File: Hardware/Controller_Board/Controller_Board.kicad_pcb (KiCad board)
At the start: 6 copper layers, 85 x 85 mm, 261 parts, among them J601 USB-C, Q101 DMN2400UFB-7, SW301 Reset, U101 TPS82084, U102 LT8645S, U103 TDS5311P, U104 TPS82084, U105 TPS82084, U106 XT30, U201 XC7A35T-CSG324, U301 IS25LP256D, U401 FT232H, U402 93LC56B, U501 FT232H, U502 93LC56B, U601 ESD122, U602 USB2512B, U701 RJ45, U702 RJ45, U703 RJ45, U704 TPD4E02B04, U705 TPD4E02B04, U706 TPD4E02B04, U710 RJ45, U711 RJ45, U712 RJ45, U713 TPD4E02B04, U714 TPD4E02B04, U715 TPD4E02B04, U716 RJ45, U717 RJ45, U718 RJ45, U719 TPD4E02B04, U720 TPD4E02B04, U721 TPD4E02B04, U722 TPD4E02B04, U723 TPD4E02B04, U724 TPD4E02B04, U725 TPD4E02B04, U726 TPD4E02B04, U727 TPD4E02B04, U728 TPD4E02B04, U729 TPD4E02B04, U730 TPD4E02B04, Y1 24MHz, Y2 12MHz, Y3 12MHz, Y301 12MHz

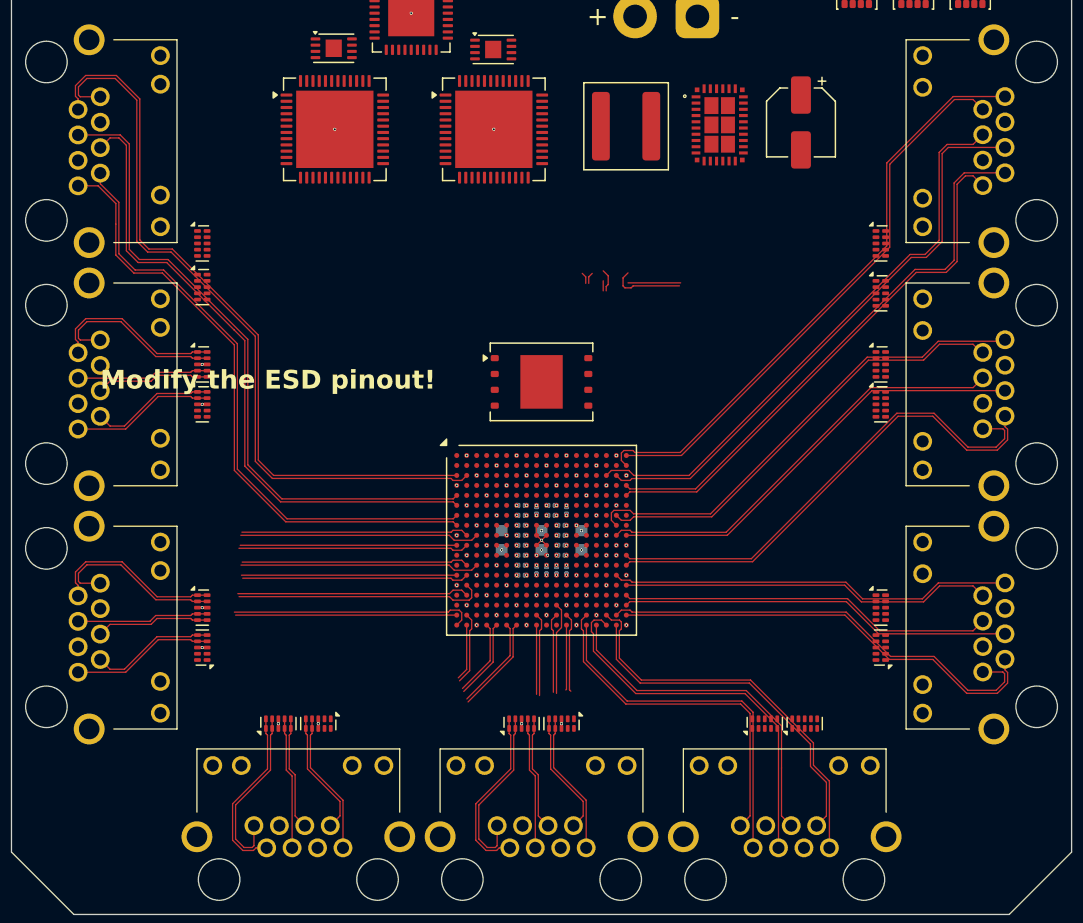
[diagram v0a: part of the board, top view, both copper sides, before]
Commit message: Commiting PCB design with 45 degree tracks
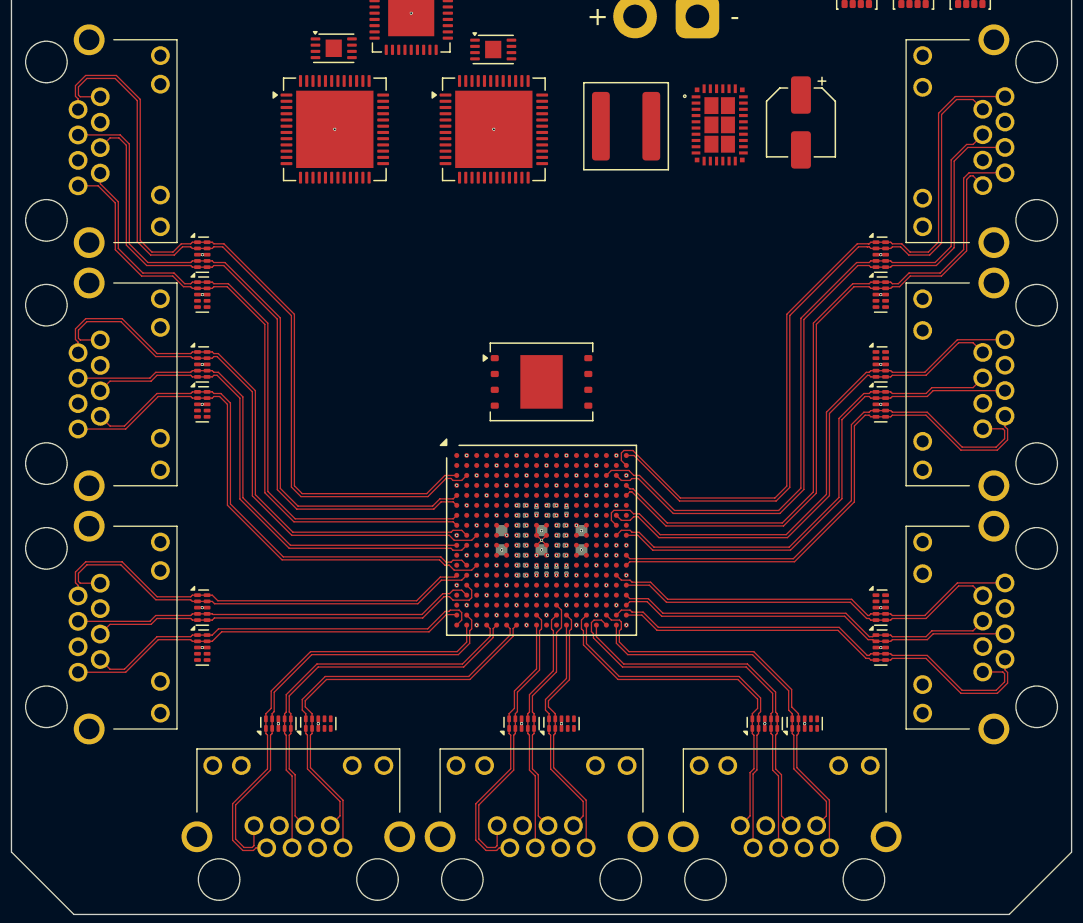
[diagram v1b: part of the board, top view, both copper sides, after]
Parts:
- moved U706 0.90 mm to (129.0, 90.3)
- moved U724 0.90 mm to (183.4, 90.3)
- moved U729 0.60 mm to (129.0, 93.5)
- moved U721 0.10 mm to (183.4, 93.5)
- turned U719 to 0 degrees
- turned U723 to 90 degrees
- turned U725 to 0 degrees
- turned U727 to 90 degrees
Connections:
- U713 pad 1: /Connectivity/P2_RX_N -> /Connectivity/P2_CLK_P
- U713 pad 10: /Connectivity/P2_RX_N -> /Connectivity/P2_CLK_P
- U713 pad 2: /Connectivity/P2_RX_P -> /Connectivity/P2_CLK_N
- U713 pad 4: /Connectivity/P2_TX_N -> /Connectivity/P2_TX_P
- U713 pad 5: /Connectivity/P2_TX_P -> /Connectivity/P2_TX_N
- U713 pad 6: /Connectivity/P2_TX_P -> /Connectivity/P2_TX_N
- U713 pad 7: /Connectivity/P2_TX_N -> /Connectivity/P2_TX_P
- U713 pad 9: /Connectivity/P2_RX_P -> /Connectivity/P2_CLK_N
- U714 pad 1: /Connectivity/P5_RX_N -> /Connectivity/P5_TX_P
- U714 pad 10: /Connectivity/P5_RX_N -> /Connectivity/P5_TX_P
- U714 pad 2: /Connectivity/P5_RX_P -> /Connectivity/P5_TX_N
- U714 pad 4: /Connectivity/P5_TX_N -> /Connectivity/P5_CLK_N
- U714 pad 5: /Connectivity/P5_TX_P -> /Connectivity/P5_CLK_P
- U714 pad 6: /Connectivity/P5_TX_P -> /Connectivity/P5_CLK_P
- U714 pad 7: /Connectivity/P5_TX_N -> /Connectivity/P5_CLK_N
- U714 pad 9: /Connectivity/P5_RX_P -> /Connectivity/P5_TX_N
- U715 pad 4: /Connectivity/P8_TX_N -> unconnected-(U715-IN-Pad4)
- U715 pad 5: /Connectivity/P8_TX_P -> unconnected-(U715-IN-Pad5)
- U715 pad 6: /Connectivity/P8_TX_P -> unconnected-(U715-NC-Pad6)
- U715 pad 7: /Connectivity/P8_TX_N -> unconnected-(U715-NC-Pad7)
- U719 pad 1: /Connectivity/P3_TX_N -> /Connectivity/P3_CLK_P
- U719 pad 10: /Connectivity/P3_TX_N -> /Connectivity/P3_CLK_P
- U719 pad 2: /Connectivity/P3_TX_P -> /Connectivity/P3_CLK_N
- U719 pad 4: /Connectivity/P3_CLK_N -> /Connectivity/P3_TX_P
- U719 pad 5: /Connectivity/P3_CLK_P -> /Connectivity/P3_TX_N
- U719 pad 6: /Connectivity/P3_CLK_P -> /Connectivity/P3_TX_N
- U719 pad 7: /Connectivity/P3_CLK_N -> /Connectivity/P3_TX_P
- U719 pad 9: /Connectivity/P3_TX_P -> /Connectivity/P3_CLK_N
- U720 pad 1: /Connectivity/P6_TX_P -> /Connectivity/P6_TX_N
- U720 pad 10: /Connectivity/P6_TX_P -> /Connectivity/P6_TX_N
- U720 pad 2: /Connectivity/P6_TX_N -> /Connectivity/P6_TX_P
- U720 pad 9: /Connectivity/P6_TX_N -> /Connectivity/P6_TX_P
- U721 pad 4: /Connectivity/P9_CLK_N -> unconnected-(U721-IN-Pad4)
- U721 pad 5: /Connectivity/P9_CLK_P -> unconnected-(U721-IN-Pad5)
- U721 pad 6: /Connectivity/P9_CLK_P -> unconnected-(U721-NC-Pad6)
- U721 pad 7: /Connectivity/P9_CLK_N -> unconnected-(U721-NC-Pad7)
- U722 pad 4: /Connectivity/P3_RX_N -> /Connectivity/P3_RX_P
- U722 pad 5: /Connectivity/P3_RX_P -> /Connectivity/P3_RX_N
- U722 pad 6: /Connectivity/P3_RX_P -> /Connectivity/P3_RX_N
- U722 pad 7: /Connectivity/P3_RX_N -> /Connectivity/P3_RX_P
- U723 pad 1: unconnected-(U723-IN-Pad1) -> /Connectivity/P6_RX_N
- U723 pad 10: unconnected-(U723-NC-Pad10) -> /Connectivity/P6_RX_N
- U723 pad 2: unconnected-(U723-IN-Pad2) -> /Connectivity/P6_RX_P
- U723 pad 4: /Connectivity/P6_RX_P -> unconnected-(U723-IN-Pad4)
- U723 pad 5: /Connectivity/P6_RX_N -> unconnected-(U723-IN-Pad5)
- U723 pad 6: /Connectivity/P6_RX_N -> unconnected-(U723-NC-Pad6)
- U723 pad 7: /Connectivity/P6_RX_P -> unconnected-(U723-NC-Pad7)
- U723 pad 9: unconnected-(U723-NC-Pad9) -> /Connectivity/P6_RX_P
- U724 pad 1: unconnected-(U724-IN-Pad1) -> /Connectivity/P9_RX_P
- U724 pad 10: unconnected-(U724-NC-Pad10) -> /Connectivity/P9_RX_P
- U724 pad 2: unconnected-(U724-IN-Pad2) -> /Connectivity/P9_RX_N
- U724 pad 4: /Connectivity/P9_RX_N -> /Connectivity/P9_CLK_P
- U724 pad 5: /Connectivity/P9_RX_P -> /Connectivity/P9_CLK_N
- U724 pad 6: /Connectivity/P9_RX_P -> /Connectivity/P9_CLK_N
- U724 pad 7: /Connectivity/P9_RX_N -> /Connectivity/P9_CLK_P
- U724 pad 9: unconnected-(U724-NC-Pad9) -> /Connectivity/P9_RX_N
- U725 pad 1: unconnected-(U725-IN-Pad1) -> /Connectivity/P1_RX_N
- U725 pad 10: unconnected-(U725-NC-Pad10) -> /Connectivity/P1_RX_N
- U725 pad 2: unconnected-(U725-IN-Pad2) -> /Connectivity/P1_RX_P
- U725 pad 4: /Connectivity/P1_RX_P -> unconnected-(U725-IN-Pad4)
- U725 pad 5: /Connectivity/P1_RX_N -> unconnected-(U725-IN-Pad5)
- U725 pad 6: /Connectivity/P1_RX_N -> unconnected-(U725-NC-Pad6)
- U725 pad 7: /Connectivity/P1_RX_P -> unconnected-(U725-NC-Pad7)
- U725 pad 9: unconnected-(U725-NC-Pad9) -> /Connectivity/P1_RX_P
- U726 pad 1: /Connectivity/P2_CLK_N -> unconnected-(U726-IN-Pad1)
- U726 pad 10: /Connectivity/P2_CLK_N -> unconnected-(U726-NC-Pad10)
- U726 pad 2: /Connectivity/P2_CLK_P -> unconnected-(U726-IN-Pad2)
- U726 pad 4: unconnected-(U726-IN-Pad4) -> /Connectivity/P2_RX_P
- U726 pad 5: unconnected-(U726-IN-Pad5) -> /Connectivity/P2_RX_N
- U726 pad 6: unconnected-(U726-NC-Pad6) -> /Connectivity/P2_RX_N
- U726 pad 7: unconnected-(U726-NC-Pad7) -> /Connectivity/P2_RX_P
- U726 pad 9: /Connectivity/P2_CLK_P -> unconnected-(U726-NC-Pad9)
- U727 pad 1: unconnected-(U727-IN-Pad1) -> /Connectivity/P4_RX_N
- U727 pad 10: unconnected-(U727-NC-Pad10) -> /Connectivity/P4_RX_N
- U727 pad 2: unconnected-(U727-IN-Pad2) -> /Connectivity/P4_RX_P
- U727 pad 4: /Connectivity/P4_RX_P -> unconnected-(U727-IN-Pad4)
- U727 pad 5: /Connectivity/P4_RX_N -> unconnected-(U727-IN-Pad5)
- U727 pad 6: /Connectivity/P4_RX_N -> unconnected-(U727-NC-Pad6)
- U727 pad 7: /Connectivity/P4_RX_P -> unconnected-(U727-NC-Pad7)
- U727 pad 9: unconnected-(U727-NC-Pad9) -> /Connectivity/P4_RX_P
- U728 pad 1: /Connectivity/P5_CLK_N -> /Connectivity/P5_RX_N
- U728 pad 10: /Connectivity/P5_CLK_N -> /Connectivity/P5_RX_N
- U728 pad 2: /Connectivity/P5_CLK_P -> /Connectivity/P5_RX_P
- U728 pad 9: /Connectivity/P5_CLK_P -> /Connectivity/P5_RX_P
- U729 pad 1: unconnected-(U729-IN-Pad1) -> /Connectivity/P7_RX_N
- U729 pad 10: unconnected-(U729-NC-Pad10) -> /Connectivity/P7_RX_N
- U729 pad 2: unconnected-(U729-IN-Pad2) -> /Connectivity/P7_RX_P
- U729 pad 4: /Connectivity/P7_RX_N -> unconnected-(U729-IN-Pad4)
- U729 pad 5: /Connectivity/P7_RX_P -> unconnected-(U729-IN-Pad5)
- U729 pad 6: /Connectivity/P7_RX_P -> unconnected-(U729-NC-Pad6)
- U729 pad 7: /Connectivity/P7_RX_N -> unconnected-(U729-NC-Pad7)
- U729 pad 9: unconnected-(U729-NC-Pad9) -> /Connectivity/P7_RX_P
- U730 pad 1: /Connectivity/P8_CLK_N -> /Connectivity/P8_TX_N
- U730 pad 10: /Connectivity/P8_CLK_N -> /Connectivity/P8_TX_N
- U730 pad 2: /Connectivity/P8_CLK_P -> /Connectivity/P8_TX_P
- U730 pad 4: unconnected-(U730-IN-Pad4) -> /Connectivity/P8_CLK_N
- U730 pad 5: unconnected-(U730-IN-Pad5) -> /Connectivity/P8_CLK_P
- U730 pad 6: unconnected-(U730-NC-Pad6) -> /Connectivity/P8_CLK_P
- U730 pad 7: unconnected-(U730-NC-Pad7) -> /Connectivity/P8_CLK_N
- U730 pad 9: /Connectivity/P8_CLK_P -> /Connectivity/P8_TX_P
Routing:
- net /Connectivity/P8_TX_P: track 19.2 -> 47.1 mm
- net /Connectivity/P8_TX_N: track 18.3 -> 46.0 mm
- net /Connectivity/P8_CLK_N: track 17.4 -> 41.1 mm
- net /Connectivity/P8_CLK_P: track 18.5 -> 40.7 mm
- net /Connectivity/P6_TX_N: track 18.4 -> 35.2 mm
- net /Connectivity/P6_TX_P: track 19.9 -> 36.3 mm
- net /Connectivity/P6_CLK_N: track 16.7 -> 31.9 mm
- net /Connectivity/P6_CLK_P: track 15.5 -> 30.4 mm
- net /Connectivity/P6_RX_N: track 17.5 -> 31.4 mm
- net /Connectivity/P9_RX_P: track 47.8 -> 61.7 mm
- net /Connectivity/P9_RX_N: track 44.6 -> 58.5 mm
- net /Connectivity/P6_RX_P: track 19.3 -> 33.0 mm
- net /Connectivity/P8_RX_N: track 28.3 -> 41.5 mm
- net /Connectivity/P8_RX_P: track 30.7 -> 43.8 mm
- net /Connectivity/P1_TX_P: track 46.7 -> 36.1 mm
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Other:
- board text removed: "Modify the ESD pinout!"
